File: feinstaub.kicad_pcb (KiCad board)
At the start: 2 copper layers, 67.1 x 62.2 mm, 14 parts, among them J1 Conn_01x04, J2 Conn_01x04, J3 Conn_01x02, SW1 SW_DIP_x01, U1 ESP-12F, U2 bme280_module, U3 AMS1117-3.3

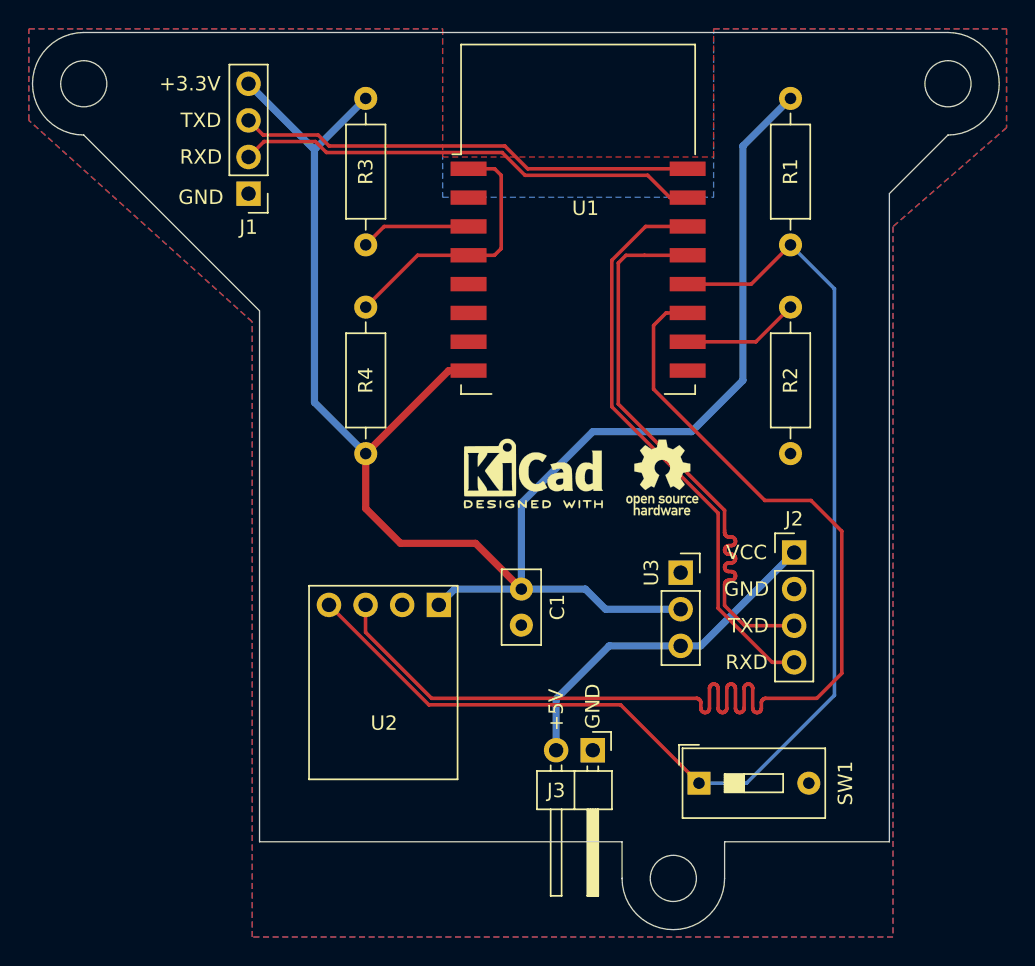
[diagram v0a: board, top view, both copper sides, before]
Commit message: small update
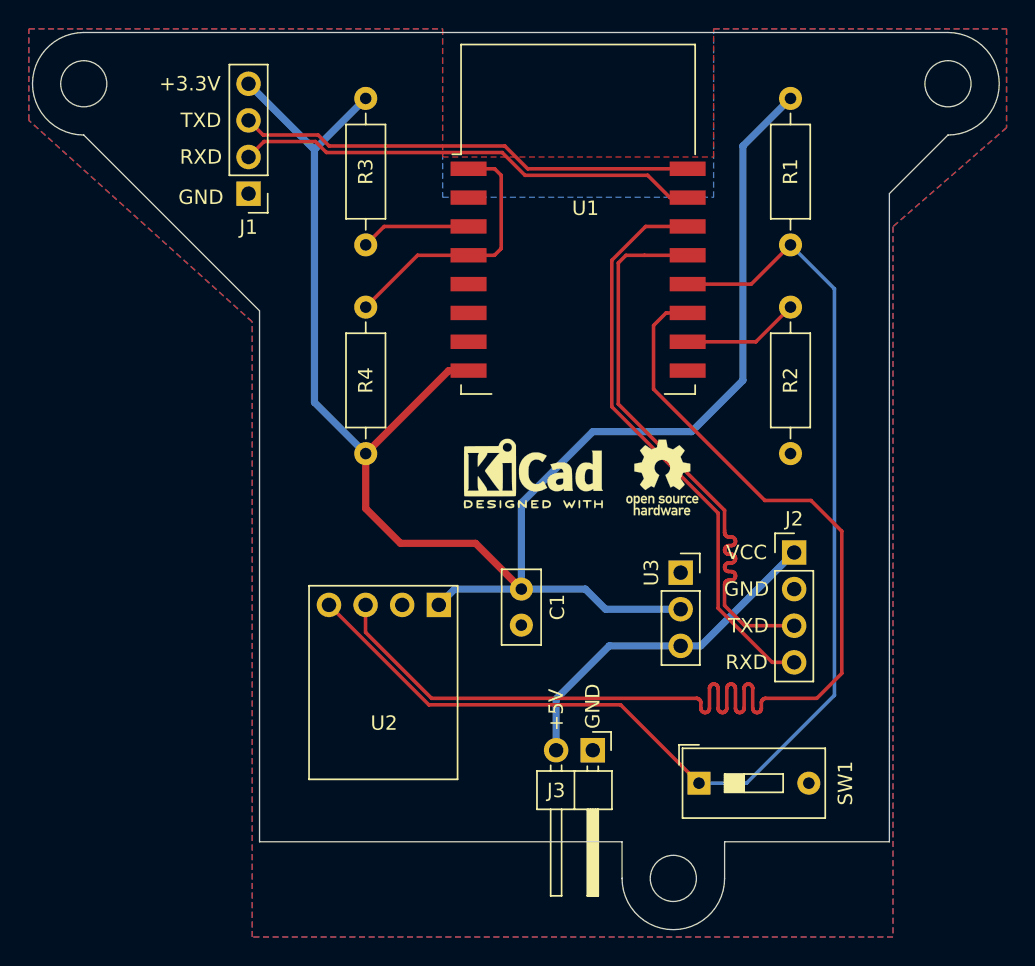
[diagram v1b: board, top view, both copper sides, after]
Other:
- net class Default removed
- net class Power removed
